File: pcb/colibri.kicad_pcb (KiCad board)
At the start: 2 copper layers, 160 x 94.7 mm, 93 parts

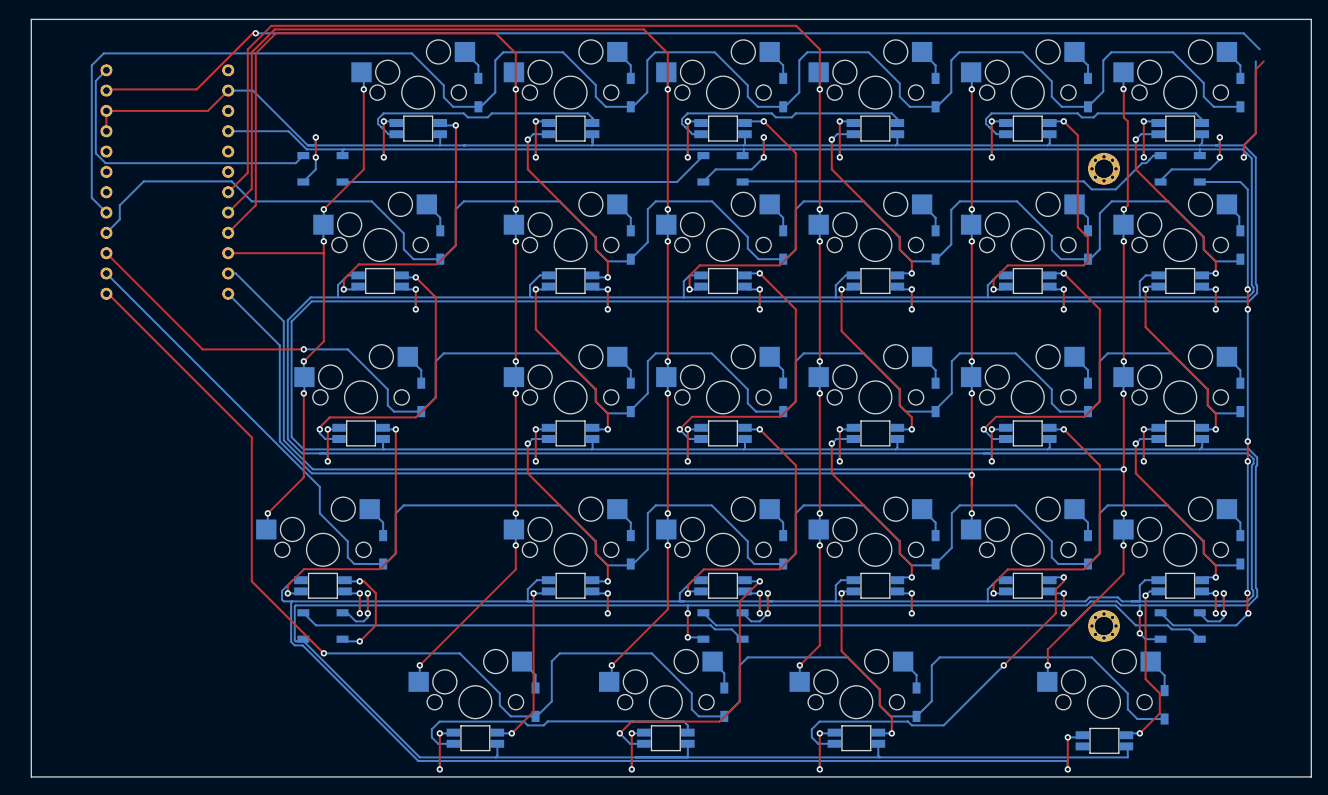
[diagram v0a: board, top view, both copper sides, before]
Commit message: board size
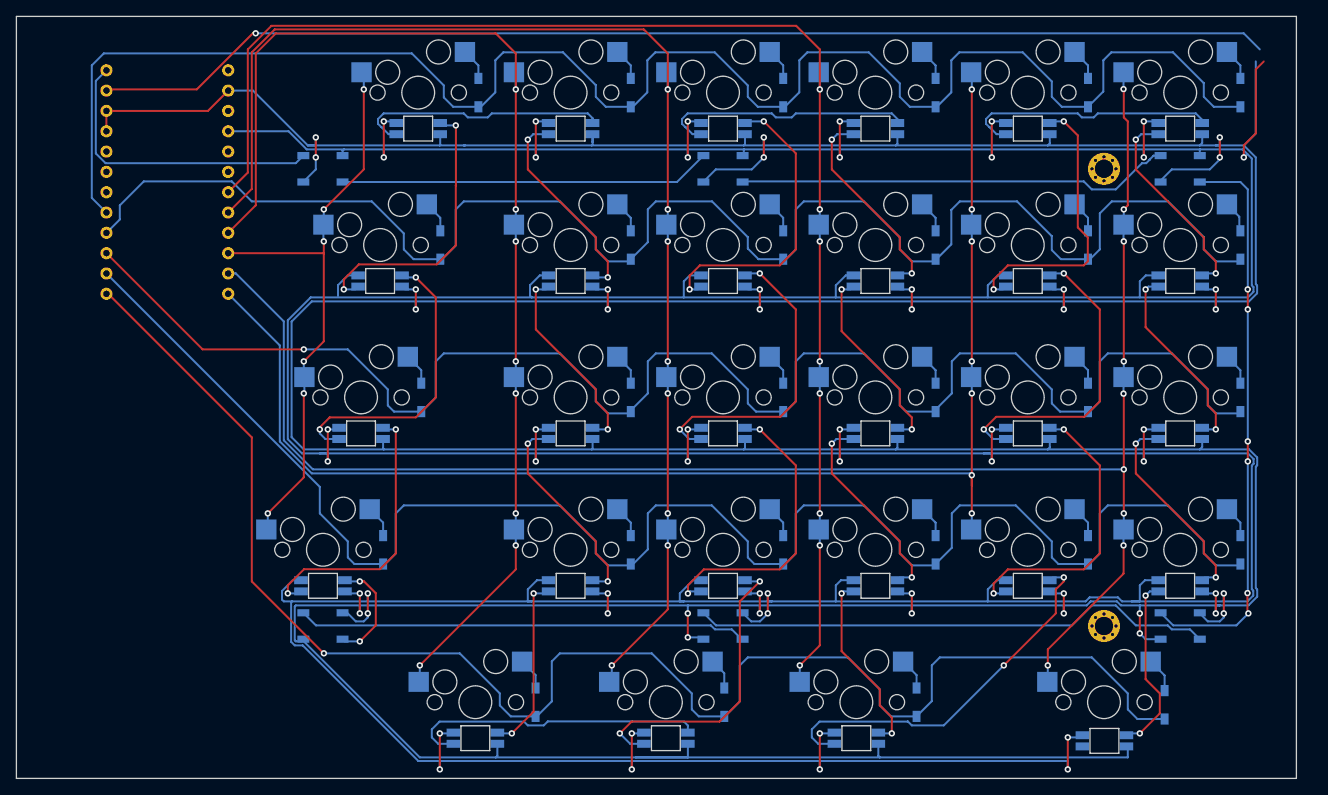
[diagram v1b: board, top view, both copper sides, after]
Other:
- board size 160 x 94.7 mm -> 160 x 95.2 mm
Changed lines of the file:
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@@
     )
   )
-  (gr_rect (start 20.440307 40.249403) (end 180.440307 134.945879) (layer "Edge.Cuts") (width 0.1) (fill none))
+  (gr_line (start 178.575 135.125) (end 18.575 135.125) (layer "Edge.Cuts") (width 0.1))
+  (gr_line (start 178.575 39.875) (end 18.575 39.875) (layer "Edge.Cuts") (width 0.1))
+  (gr_line (start 18.575 39.875) (end 18.575 135.125) (layer "Edge.Cuts") (width 0.1))
+  (gr_line (start 178.575 39.875) (end 178.575 135.125) (layer "Edge.Cuts") (width 0.1))
   (segment (start 91 49.924905) (end 91 48.462452) (width 0.25) (layer "B.Cu") (net 1))
   (segment (start 73.175 51.175) (end 72 50) (width 0.25) (layer "B.Cu") (net 1))
